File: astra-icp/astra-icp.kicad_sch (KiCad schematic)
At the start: 70 parts, among them IC1 ATA6561-GAQW-N, J1 PINHD_1x5_Male, J2 PWR_IN, J3 CAN_TERMINAL, SW1 CHOC_HS, SW10 CHOC_HS, SW11 CHOC_HS, SW12 CHOC_HS, SW13 CHOC_HS, SW14 CHOC_HS, SW15 CHOC_HS, SW16 CHOC_HS, SW17 CHOC_HS, SW18 CHOC_HS, SW19 CHOC_HS, SW2 CHOC_HS, SW20 CHOC_HS, SW3 CHOC_HS, SW4 CHOC_HS, SW5 CHOC_HS, SW6 CHOC_HS, SW7 CHOC_HS, SW8 CHOC_HS, SW9 CHOC_HS, U3 STM32F042C4Tx

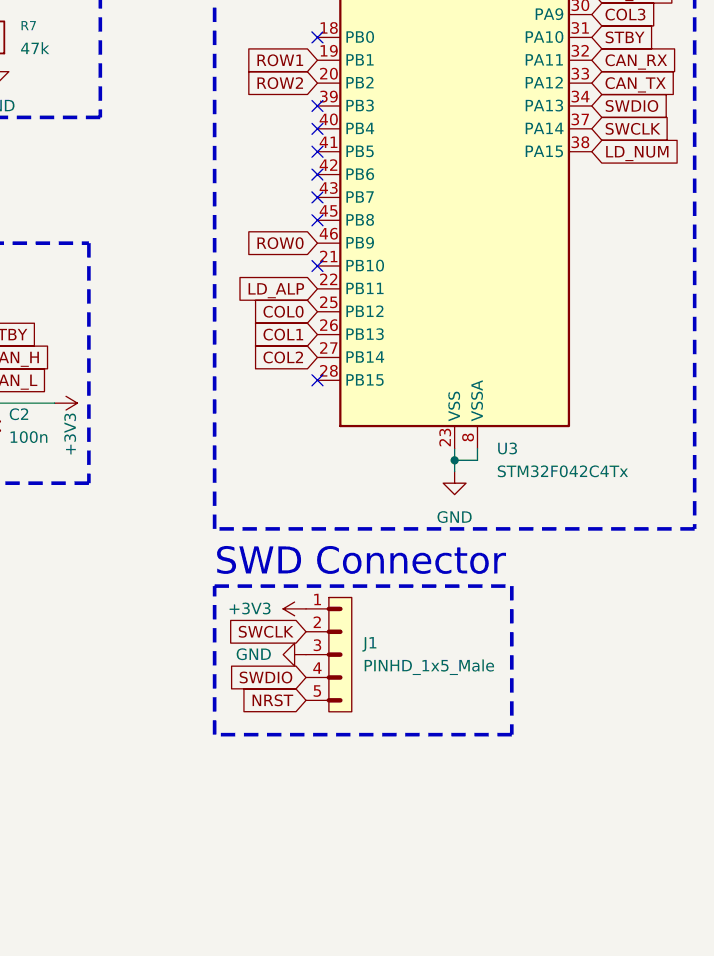
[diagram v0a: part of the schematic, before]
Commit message: feat: Final work on ICP PCB
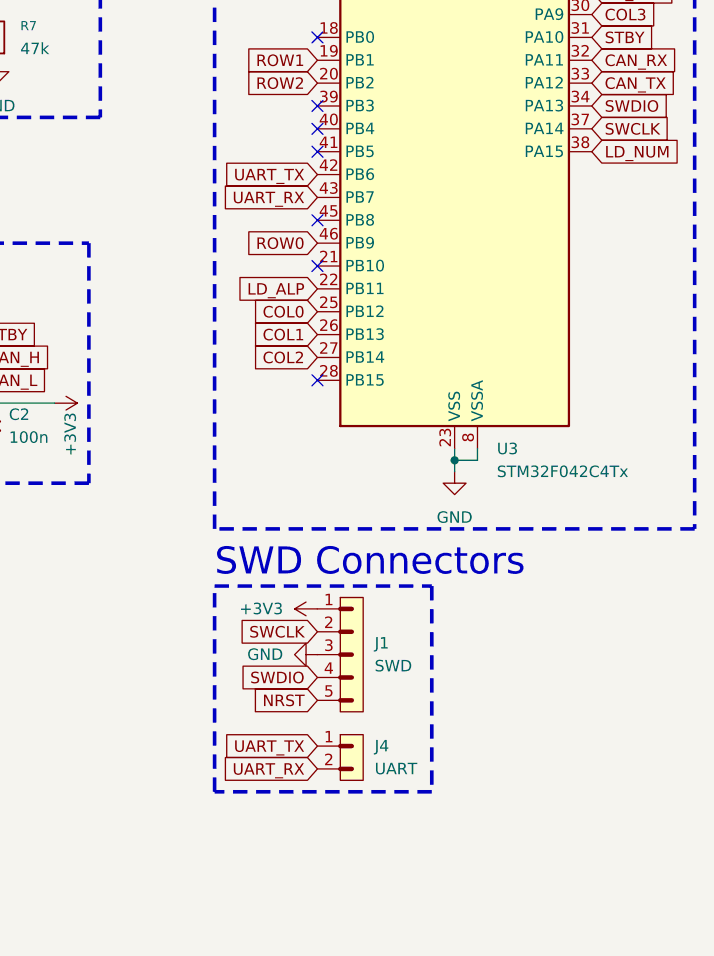
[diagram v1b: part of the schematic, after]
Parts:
- added J4: UART, Connector_PinHeader_2.54mm:PinHeader_1x02_P2.54mm_Vertical, symbol PCM_SL_Pin_Headers:PINHD_1x2_Male
- J1: value PINHD_1x5_Male -> SWD
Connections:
- net UART_TX: now reaches U3.42 (PB6)
- net UART_TX: now also J4.1
- net UART_RX: now reaches U3.43 (PB7)
- net UART_RX: now also J4.2
- no-connect marks 16 -> 14
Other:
- note added: "SWD Connectors"
- note removed: "SWD Connector"
- moved on the sheet: J1
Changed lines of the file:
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@@
 	(rectangle
 		(start 165.1 127)
-		(end 198.12 143.51)
+		(end 189.23 149.86)
 		(stroke
 			(width 0.4)
@@
 		)
 	)
-	(text "SWD Connector"
+	(text "SWD Connectors"
 		(exclude_from_sim no)
 		(at 165.1 124.46 0)
@@
 	)
 	(no_connect
-		(at 176.53 81.28)
+		(at 176.53 73.66)
 	)
 	(no_connect
@@
 	)
 	(no_connect
-		(at 176.53 78.74)
+		(at 176.53 86.36)
 	)
 	(no_connect
-		(at 176.53 58.42)
+		(at 176.53 78.74)
 	)
 	(no_connect
-		(at 176.53 83.82)
+		(at 176.53 58.42)
 	)
 	(no_connect
@@
 	)
 	(no_connect
-		(at 176.53 104.14)
-	)
-	(no_connect
-		(at 176.53 73.66)
+		(at 176.53 76.2)
 	)
 	(no_connect
-		(at 176.53 76.2)
+		(at 176.53 104.14)
 	)
 	(no_connect
@@
 		(at 176.53 60.96)
 	)
-	(no_connect
-		(at 176.53 86.36)
-	)
 	(wire
 		(pts
@@
 		)
 	)
+	(global_label "UART_TX"
+		(shape input)
+		(at 176.53 81.28 180)
+		(fields_autoplaced yes)
+		(effects
+			(font
+				(size 1.27 1.27)
+			)
+			(justify right)
+		)
+		(property "Intersheetrefs" "${INTERSHEET_REFS}"
+			(at 165.7434 81.28 0)
+			(effects
+				(font
+					(size 1.27 1.27)
+				)
+				(justify right)
+				(hide yes)
+			)
+		)
+	)
 	(global_label "SWDIO"
 		(shape input)
@@
 	(global_label "NRST"
 		(shape input)
-		(at 175.26 139.7 180)
+		(at 176.53 139.7 180)
 		(fields_autoplaced yes)
 		(effects
@@
 		)
 		(property "Intersheetrefs" "${INTERSHEET_REFS}"
-			(at 167.4972 139.7 0)
+			(at 168.7672 139.7 0)
 			(effects
 				(font
@@
 		)
 	)
+	(global_label "UART_TX"
+		(shape input)
+		(at 176.53 144.78 180)
+		(fields_autoplaced yes)
+		(effects
+			(font
+				(size 1.27 1.27)
+			)
+			(justify right)
+		)
+		(property "Intersheetrefs" "${INTERSHEET_REFS}"
+			(at 165.7434 144.78 0)
+			(effects
+				(font
+					(size 1.27 1.27)
+				)
+				(justify right)
+				(hide yes)
+			)
+		)
+	)
 	(global_label "SWCLK"
 		(shape input)
@@
 	(global_label "SWCLK"
 		(shape input)
-		(at 175.26 132.08 180)
+		(at 176.53 132.08 180)
 		(fields_autoplaced yes)
 		(effects
@@
 		)
 		(property "Intersheetrefs" "${INTERSHEET_REFS}"
-			(at 166.0458 132.08 0)
+			(at 167.3158 132.08 0)
 			(effects
 				(font
@@
 		)
 	)
+	(global_label "UART_RX"
+		(shape input)
+		(at 176.53 147.32 180)
+		(fields_autoplaced yes)
+		(effects
+			(font
+				(size 1.27 1.27)
+			)
+			(justify right)
+		)
+		(property "Intersheetrefs" "${INTERSHEET_REFS}"
+			(at 165.441 147.32 0)
+			(effects
+				(font
+					(size 1.27 1.27)
+				)
+				(justify right)
+				(hide yes)
+			)
+		)
+	)
 	(global_label "ROW5"
 		(shape input)
@@
 		)
 	)
+	(global_label "UART_RX"
+		(shape input)
+		(at 176.53 83.82 180)
+		(fields_autoplaced yes)
+		(effects
+			(font
+				(size 1.27 1.27)
+			)
+			(justify right)
+		)
+		(property "Intersheetrefs" "${INTERSHEET_REFS}"
+			(at 165.441 83.82 0)
+			(effects
+				(font
+					(size 1.27 1.27)
+				)
+				(justify right)
+				(hide yes)
+			)
+		)
+	)
 	(global_label "LD_NUM"
 		(shape input)
@@
 	(global_label "SWDIO"
 		(shape input)
-		(at 175.26 137.16 180)
+		(at 176.53 137.16 180)
 		(fields_autoplaced yes)
 		(effects
@@
 		)
 		(property "Intersheetrefs" "${INTERSHEET_REFS}"
-			(at 166.4086 137.16 0)
+			(at 167.6786 137.16 0)
 			(effects
 				(font
@@
 	(symbol
 		(lib_id "power:+3V3")
-		(at 175.26 129.54 90)
+		(at 176.53 129.54 90)
 		(unit 1)
 		(exclude_from_sim no)
@@
 		(fields_autoplaced yes)
 		(property "Reference" "#PWR034"
-			(at 179.07 129.54 0)
+			(at 180.34 129.54 0)
 			(effects
 				(font
@@
 		)
 		(property "Value" "+3V3"
-			(at 171.45 129.5399 90)
+			(at 172.72 129.5399 90)
 			(effects
 				(font
@@
 		)
 		(property "Footprint" ""
-			(at 175.26 129.54 0)
+			(at 176.53 129.54 0)
 			(effects
 				(font
@@
 		)
 		(property "Datasheet" ""
-			(at 175.26 129.54 0)
+			(at 176.53 129.54 0)
 			(effects
 				(font
@@
 		)
 		(property "Description" "Power symbol creates a global label with name \"+3V3\""
-			(at 175.26 129.54 0)
+			(at 176.53 129.54 0)
 			(effects
 				(font
@@
 	(symbol
 		(lib_id "PCM_SL_Pin_Headers:PINHD_1x5_Male")
-		(at 179.07 134.62 0)
+		(at 180.34 134.62 0)
 		(unit 1)
 		(exclude_from_sim no)
@@
 		(fields_autoplaced yes)
 		(property "Reference" "J1"
-			(at 181.61 133.3499 0)
+			(at 182.88 133.3499 0)
 			(effects
 				(font
@@
 			)
 		)
-		(property "Value" "PINHD_1x5_Male"
-			(at 181.61 135.8899 0)
+		(property "Value" "SWD"
+			(at 182.88 135.8899 0)
 			(effects
 				(font
@@
 		)
 		(property "Footprint" "Connector_PinHeader_2.54mm:PinHeader_1x05_P2.54mm_Vertical"
-			(at 177.8 121.92 0)
+			(at 179.07 121.92 0)
 			(effects
 				(font
@@
 		)
 		(property "Datasheet" ""
-			(at 179.07 123.19 0)
+			(at 180.34 123.19 0)
 			(effects
 				(font
@@
 		)
 		(property "Description" "Pin Header male with pin space 2.54mm. Pin Count -5"
-			(at 179.07 134.62 0)
+			(at 180.34 134.62 0)
 			(effects
 				(font
@@
 	)
 	(symbol
+		(lib_id "PCM_SL_Pin_Headers:PINHD_1x2_Male")
+		(at 180.34 146.05 0)
+		(unit 1)
+		(exclude_from_sim no)
+		(in_bom yes)
+		(on_board yes)
+		(dnp no)
+		(fields_autoplaced yes)
+		(property "Reference" "J4"
+			(at 182.88 144.7799 0)
+			(effects
+				(font
+					(size 1.27 1.27)
+				)
+				(justify left)
+			)
+		)
+		(property "Value" "UART"
+			(at 182.88 147.3199 0)
+			(effects
+				(font
+					(size 1.27 1.27)
+				)
+				(justify left)
+			)
+		)
+		(property "Footprint" "Connector_PinHeader_2.54mm:PinHeader_1x02_P2.54mm_Vertical"
+			(at 181.61 149.86 0)
+			(effects
+				(font
+					(size 1.27 1.27)
+				)
+				(hide yes)
+			)
+		)
+		(property "Datasheet" ""
+			(at 180.34 138.43 0)
+			(effects
+				(font
+					(size 1.27 1.27)
+				)
+				(hide yes)
+			)
+		)
+		(property "Description" "Pin Header male with pin space 2.54mm. Pin Count -2"
+			(at 180.34 146.05 0)
+			(effects
+				(font
+					(size 1.27 1.27)
+				)
+				(hide yes)
+			)
+		)
+		(pin "1"
+		)
+		(pin "2"
+		)
+		(instances
+			(project ""
+				(path "/2c0b7f62-c984-4395-ba2f-356f19f7f2d0"
+					(reference "J4")
+					(unit 1)
+				)
+			)
+		)
+	)
+	(symbol
 		(lib_id "power:+5V")
 		(at 36.83 173.99 90)
@@
 	(symbol
 		(lib_id "power:GND")
-		(at 175.26 134.62 270)
+		(at 176.53 134.62 270)
 		(unit 1)
 		(exclude_from_sim no)
@@
 		(fields_autoplaced yes)
 		(property "Reference" "#PWR035"
-			(at 168.91 134.62 0)
+			(at 170.18 134.62 0)
 			(effects
 				(font
@@
 		)
 		(property "Value" "GND"
-			(at 171.45 134.6199 90)
+			(at 172.72 134.6199 90)
 			(effects
 				(font
@@
 		)
 		(property "Footprint" ""
-			(at 175.26 134.62 0)
+			(at 176.53 134.62 0)
 			(effects
 				(font
@@
 		)
 		(property "Datasheet" ""
-			(at 175.26 134.62 0)
+			(at 176.53 134.62 0)
 			(effects
 				(font
@@
 		)
 		(property "Description" "Power symbol creates a global label with name \"GND\" , ground"
-			(at 175.26 134.62 0)
+			(at 176.53 134.62 0)
 			(effects
 				(font
